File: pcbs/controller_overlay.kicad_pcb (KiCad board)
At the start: 2 copper layers, 19.7 x 60.1 mm, 2 parts

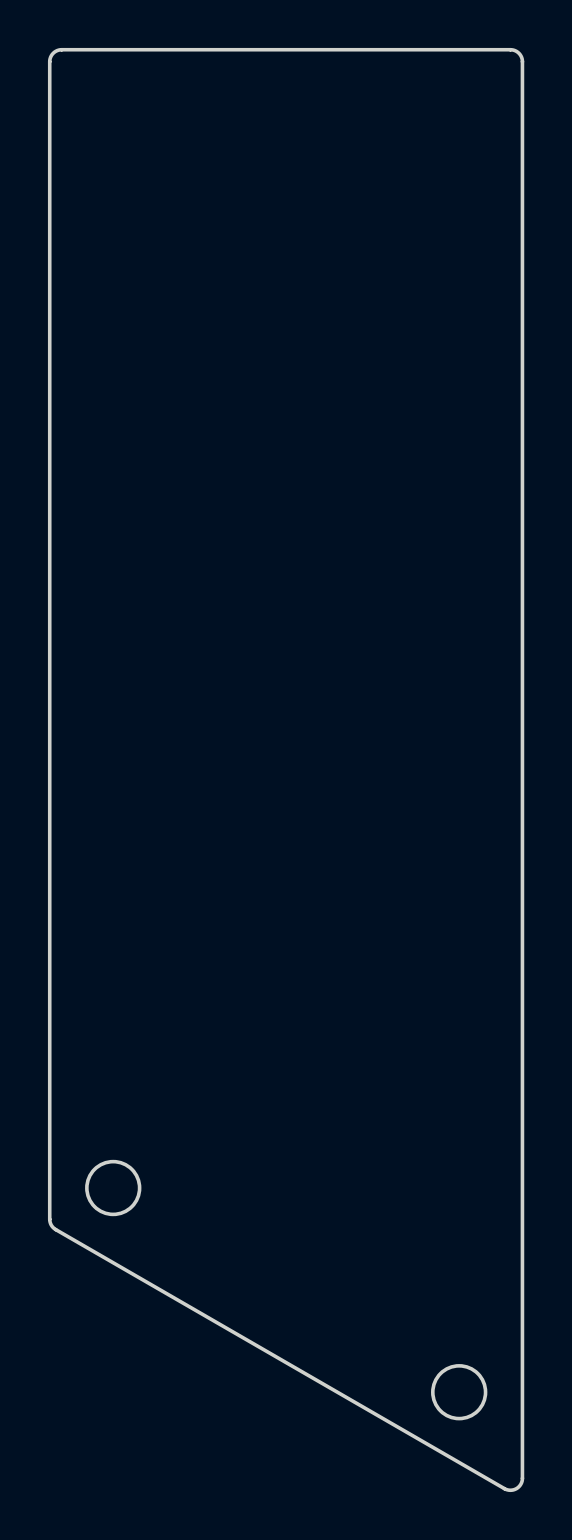
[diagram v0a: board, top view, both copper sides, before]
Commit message: build: regenerate outlines and PCBs with Ergogen snapshot
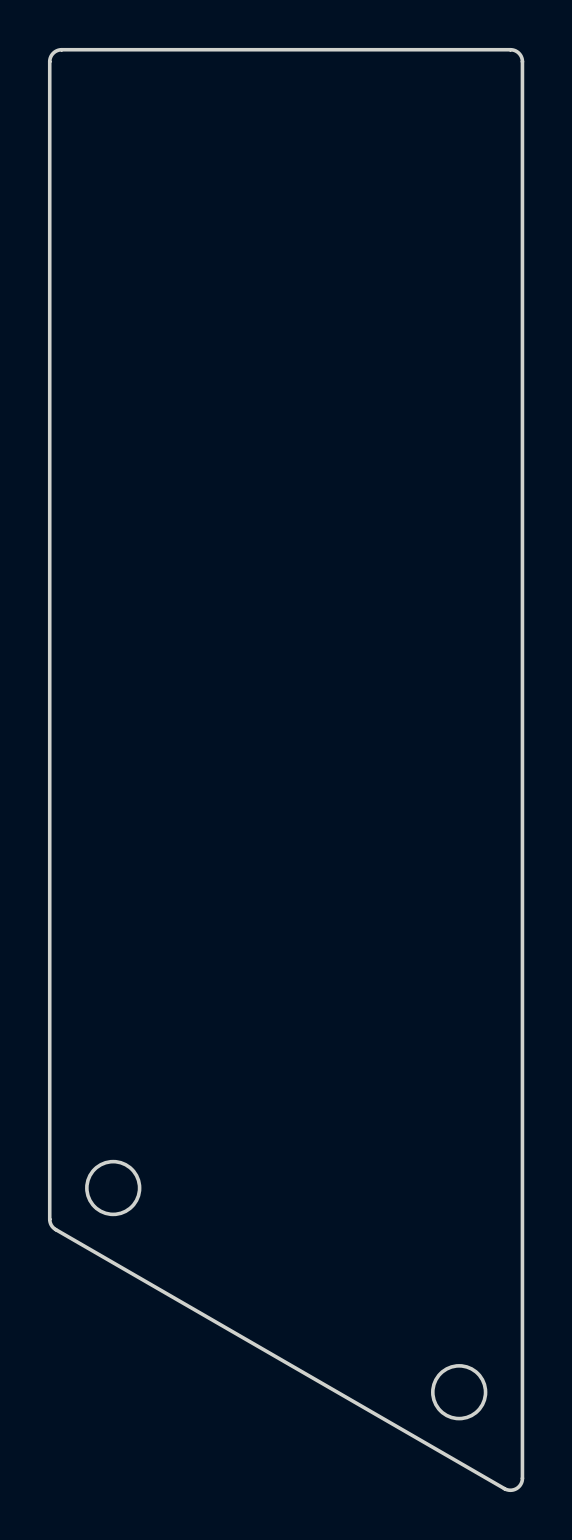
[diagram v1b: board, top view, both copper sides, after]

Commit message: build: regenerate PCBs, images, and gerbers
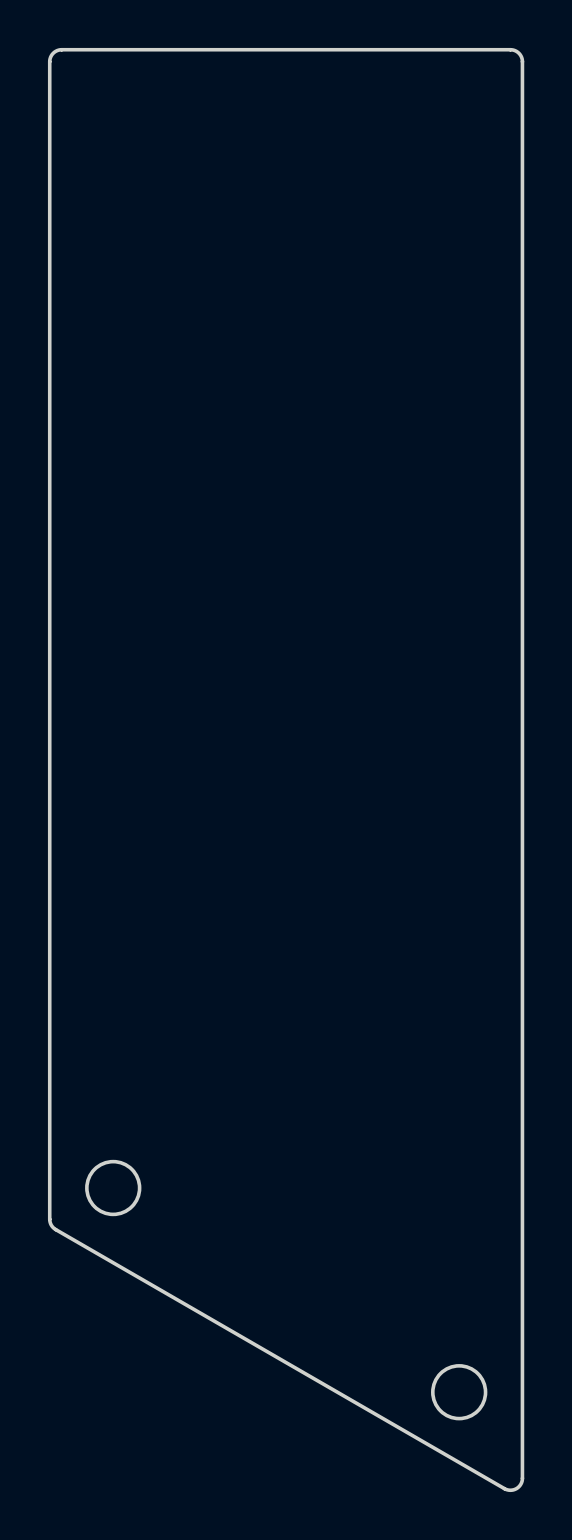
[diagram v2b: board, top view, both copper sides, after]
